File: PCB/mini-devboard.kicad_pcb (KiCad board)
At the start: 2 copper layers, 19 x 56.4 mm, 16 parts, among them J1 USB_A, J2 Conn_02x05_Counter_Clockwise, SW1 SW_Push, U1 CH552G

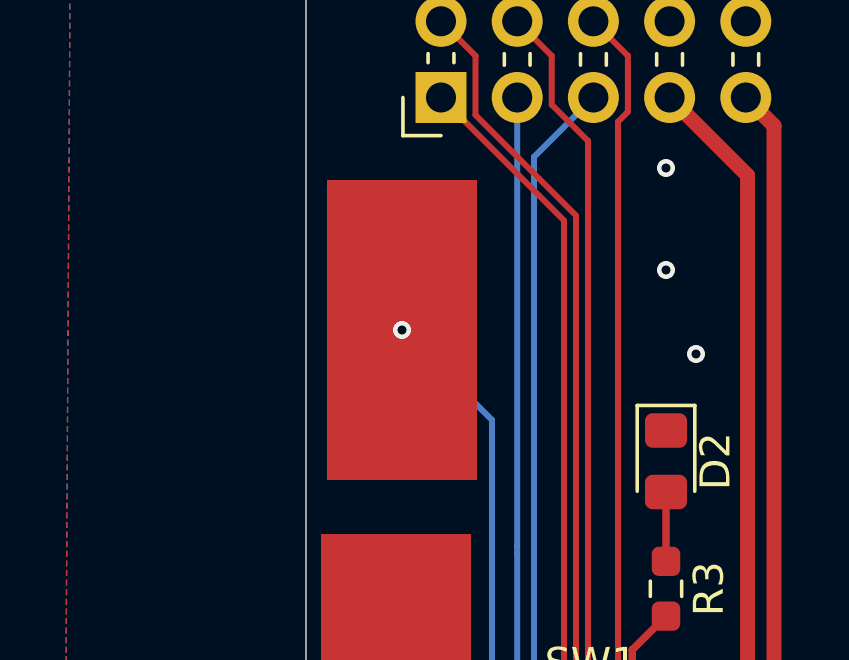
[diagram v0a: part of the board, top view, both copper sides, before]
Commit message: finishing touches
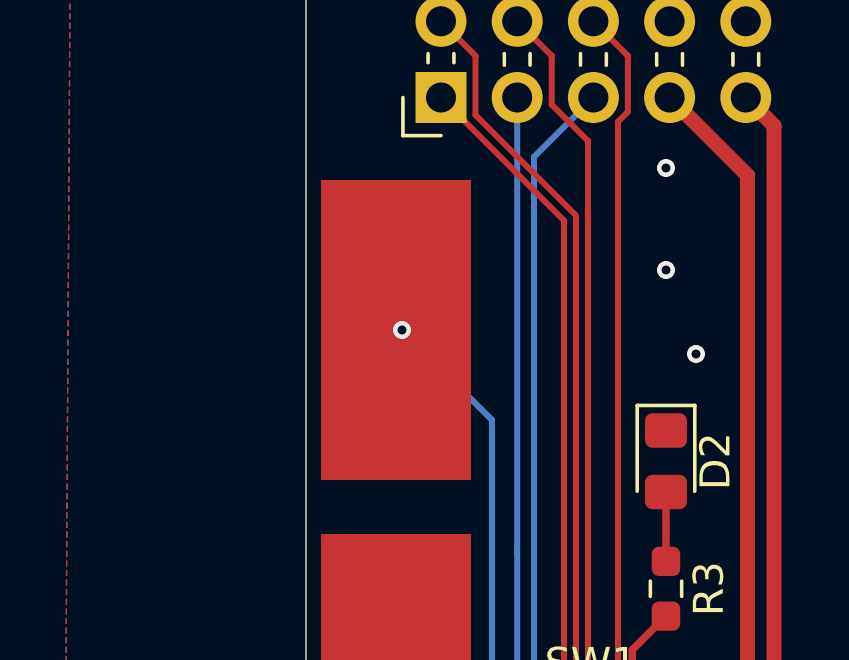
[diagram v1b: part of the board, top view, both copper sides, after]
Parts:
- moved TP2 0.20 mm to (122.0, 89.0)
